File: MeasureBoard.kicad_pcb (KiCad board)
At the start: 2 copper layers, 60 x 77 mm, 129 parts, among them J1 Conn_01x04, J10 TEST_1P, J11 TEST_1P, J12 TEST_1P, J13 BARREL_JACK, J14 CONN_01X02, J15 Conn_02x05_Odd_Even, J16 Conn_01x06, J17 GS3, J18 USB_OTG, J19 Conn_01x02, J2 Conn_01x06, J20 Conn_01x02, J21 Conn_01x03, J22 Conn_01x03, J23 Conn_01x03, J24 Conn_01x03, J25 Conn_01x03, J26 Conn_01x03, J27 Conn_02x05_Odd_Even, J3 Conn_01x04, J4 GS3, J5 GS2, J6 Conn_01x04, J7 Conn_01x03, J8 Conn_01x04, J9 TEST_1P, SW1 DIP_SW_2P, SW2 SKRPACE010, SW3 SKRPACE010, SW4 SKRPACE010, U1 L7805, U2 AP1117-33, U3 STM32F103CBTx, U4 NC7SZ08, U5 SP3481CN, U6 NC7WZ241, U7 MCP2562-E-SN, U8 AM26LV32, Y1 Crystal

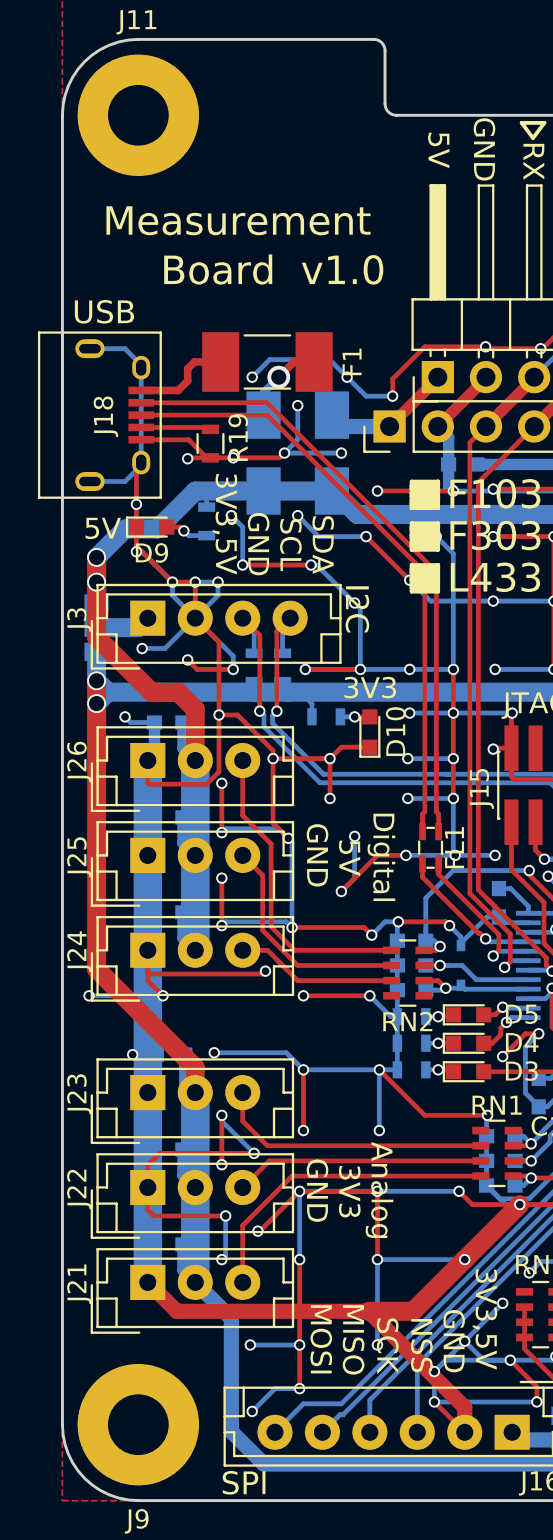
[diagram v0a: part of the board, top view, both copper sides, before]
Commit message: USBのいち変更
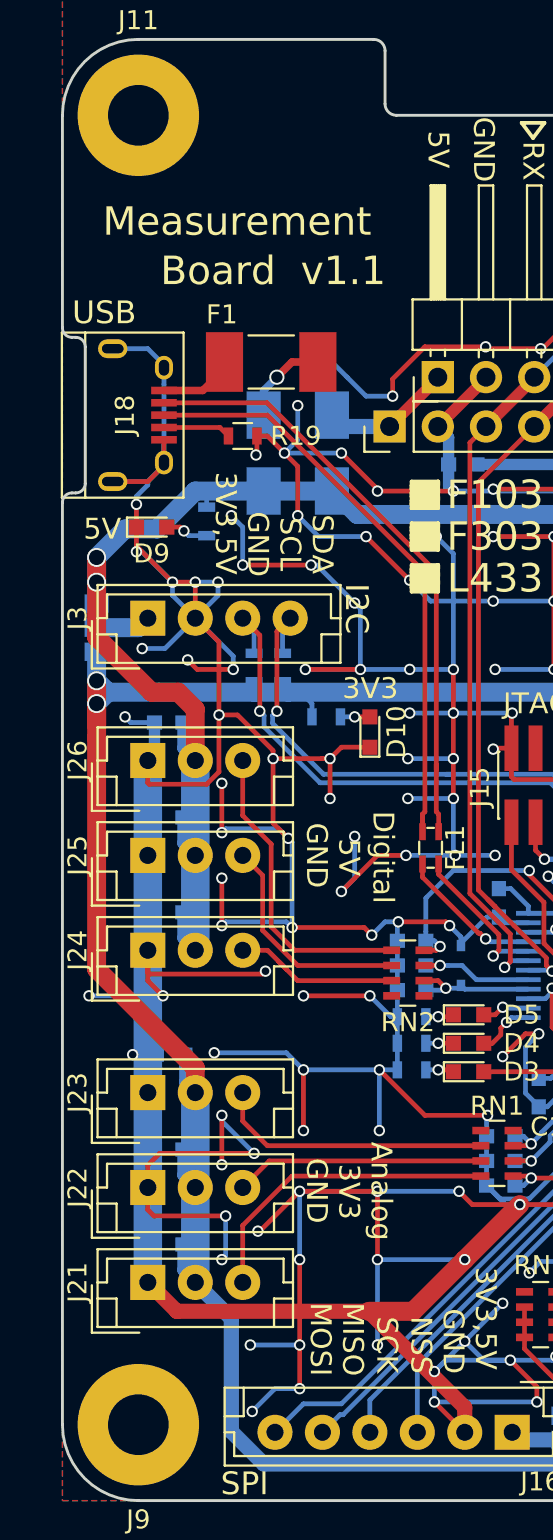
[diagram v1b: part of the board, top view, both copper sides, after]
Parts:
- moved R19 1.75 mm to (59.5, 93.9), turned to 0 degrees
- moved J18 1.20 mm to (54.0, 92.8)
- moved F1 0.20 mm to (61.0, 90.0)
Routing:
- net GND: track 1161.2 -> 1159.9 mm, vias 267 -> 264
- net Net-(FL1-Pad3): track 32.6 -> 31.4 mm
- net Net-(FL1-Pad1): track 33.3 -> 32.1 mm
- net Net-(F1-Pad2): track 5.19 -> 4.02 mm
- net Net-(D11-Pad2): track 4.52 -> 5.08 mm
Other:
- outline, holes or cut-outs redrawn
- board text added: "v1.1"
- board text removed: "v1.0"
